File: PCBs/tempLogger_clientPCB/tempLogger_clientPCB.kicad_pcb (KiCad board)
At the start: 2 copper layers, 45.7 x 61 mm, 5 parts

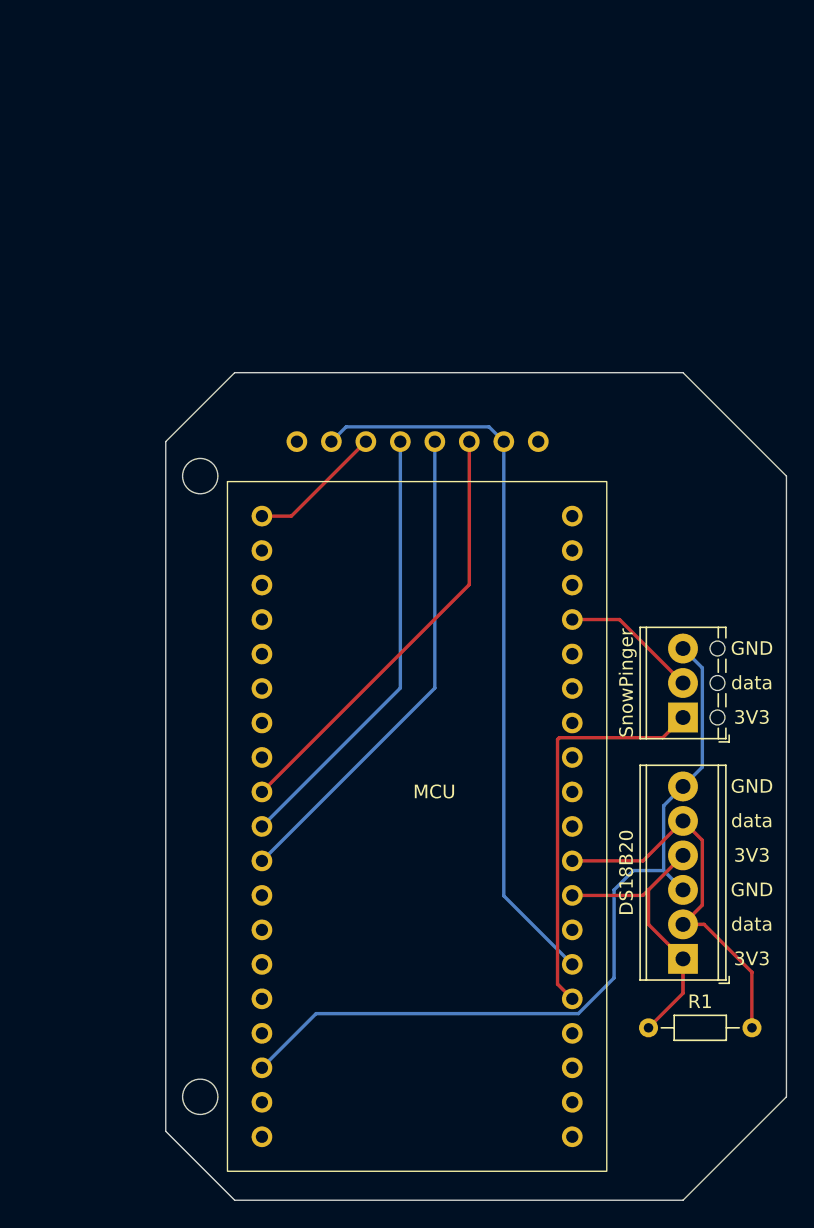
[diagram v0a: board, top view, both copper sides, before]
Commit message: mostly pcb updates. beginning of arcwatch deployment code. updates to libs
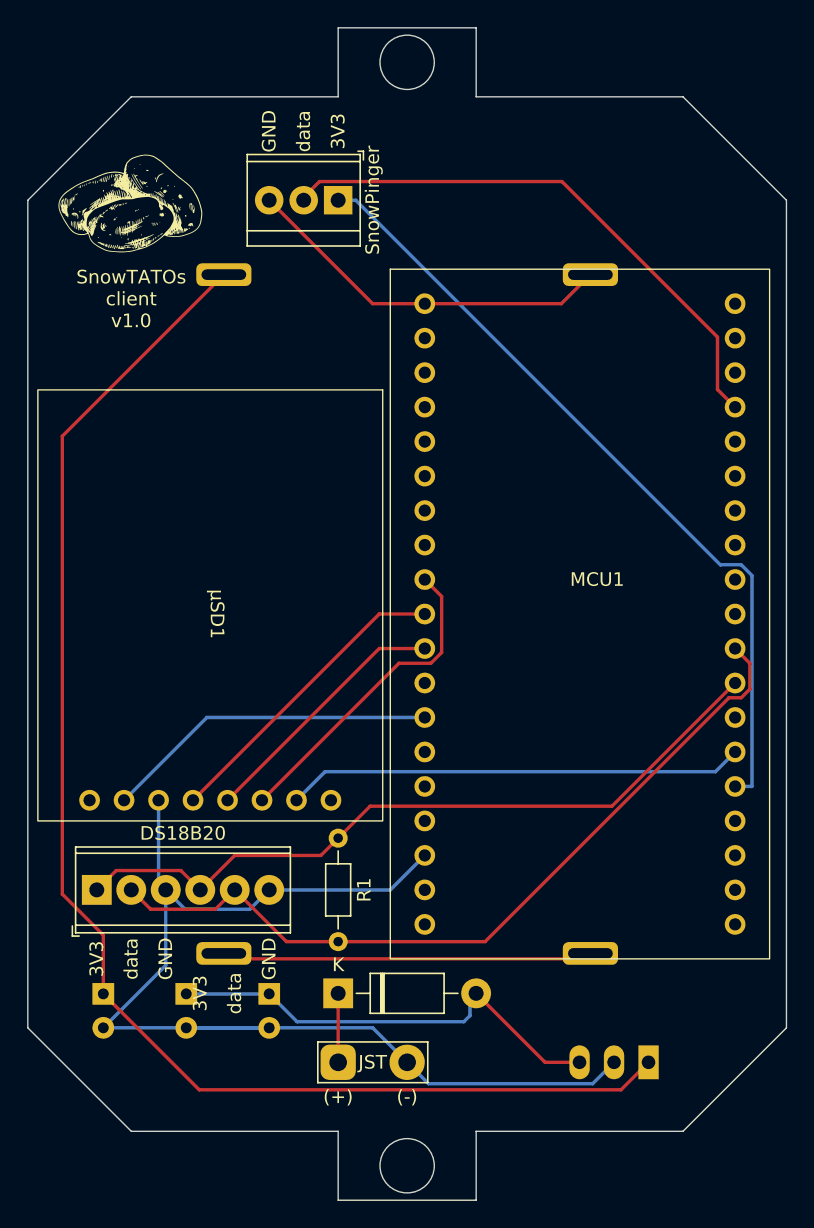
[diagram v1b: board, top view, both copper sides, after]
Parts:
- added BT1: 3.6V, Battery:battery_c_cell_solderTabs, B.Cu at (143.0, 91.4)
- added BT2: 3.6V, Battery:battery_c_cell_solderTabs, B.Cu at (116.0, 91.4)
- added C1: 10µF, Capacitor_THT:CP_Radial_Tantal_D4.5mm_P2.50mm, B.Cu at (107.2, 119.4)
- added C2: 47µF, Capacitor_THT:CP_Radial_Tantal_D4.5mm_P2.50mm, B.Cu at (113.3, 119.4)
- added C3: 47µF, Capacitor_THT:CP_Radial_Tantal_D4.5mm_P2.50mm, B.Cu at (119.4, 119.4)
- added D1: 1n5820, Diode_THT:D_DO-41_SOD81_P10.16mm_Horizontal, F.Cu at (124.5, 119.4)
- added G***: LOGO, LOGO, F.Cu at (109.2, 61.0)
- added JST1: JST male flying leads, TestPoint:TestPoint_2Pads_Pitch5.08mm_Drill1.3mm, F.Cu at (124.5, 124.5)
- added U1: TPSM84203, Converter_DCDC:Converter_DCDC_TRACO_TSR-1_THT, B.Cu at (147.3, 124.5)
- SnowPinger: footprint TerminalBlock_Phoenix:TerminalBlock_Phoenix_MPT-0,5-3-2.54_1x03_P2.54mm_Horizontal -> TerminalBlock_TE-Connectivity:TerminalBlock_TE_282834-3_1x03_P2.54mm_Horizontal
- µSD1: renamed from µSD; moved to F.Cu
- moved SnowPinger 45.8 mm to (124.5, 61.0), turned to 180 degrees
- moved DS18B20 43.5 mm to (106.7, 111.8), turned to 0 degrees
- moved R1 26.8 mm to (124.5, 108.0), turned to -90 degrees
- moved MCU1 19.7 mm to (143.5, 91.4)
- moved µSD1 14.5 mm to (115.0, 91.4), turned to -90 degrees
- renumbered MCU to MCU1
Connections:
- µSD1 pad 7: /sd_cs -> /3V3
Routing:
- net Net-(BT2-+): track 0.00 -> 103.1 mm
- net /GND: track 69.5 -> 114.0 mm
- net Net-(D1-A): track 0.00 -> 33.3 mm
- net Net-(DS18B20-Pin_1): track 21.6 -> 54.5 mm
- net Net-(MCU1-SERIAL1_RX): track 10.1 -> 41.6 mm
- net Net-(DS18B20-Pin_2): track 28.8 -> 59.5 mm
- net Net-(MCU1-D11): track 29.5 -> 58.7 mm
- net Net-(BT1-+): track 0.00 -> 27.7 mm
- net /3V3: track 0.00 -> 24.7 mm
- net /sd_cs: track 54.2 -> 33.8 mm
- net Net-(MCU1-MISO): track 36.2 -> 19.2 mm
- net Net-(MCU1-SCK): track 32.6 -> 22.8 mm
- net Net-(MCU1-MOSI): track 32.1 -> 23.6 mm
- net Net-(D1-K): track 0.00 -> 5.08 mm
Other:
- board size 45.7 x 61 mm -> 55.9 x 86.4 mm
- board text added: "(+)"
- board text added: "(-)"
- board text added: "JST"
- board text added: "SnowTATOs client v1.0"
